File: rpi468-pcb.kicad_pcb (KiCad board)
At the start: 2 copper layers, 14 x 28.3 mm, 11 parts, among them J1 USB_A, J2 USB_C_Receptacle_USB2.0, J3 Conn_01x04_Female, U1 LM397

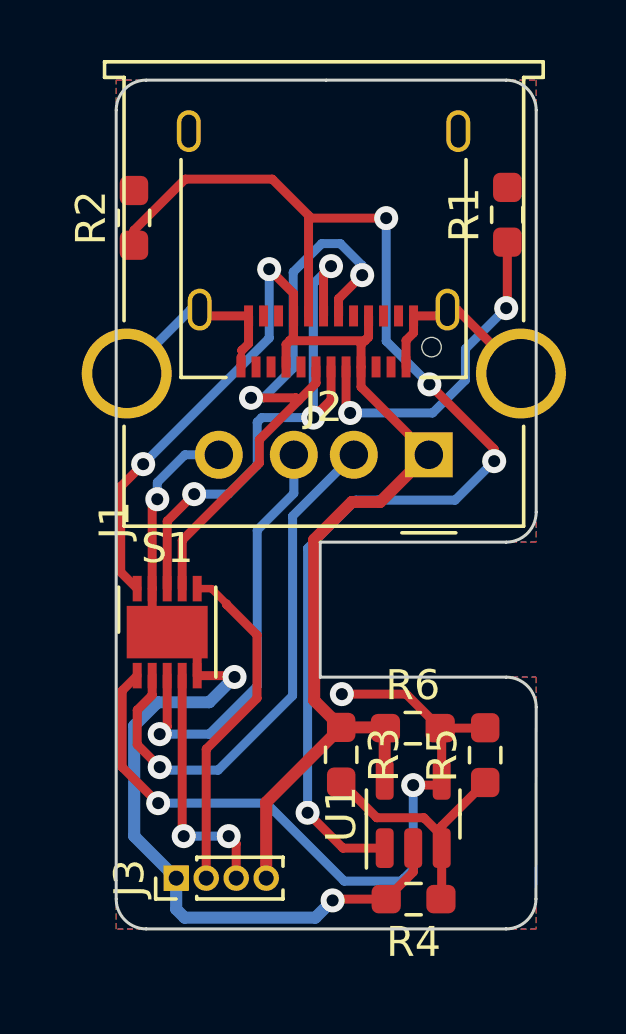
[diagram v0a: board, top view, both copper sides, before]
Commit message: some cleanup
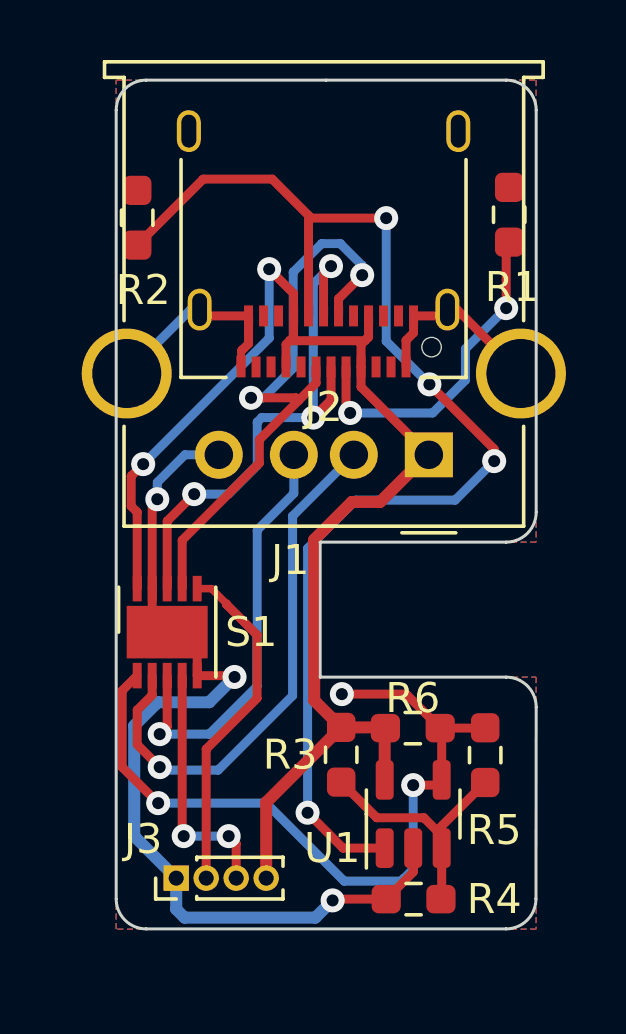
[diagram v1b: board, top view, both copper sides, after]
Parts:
- moved R2 0.11 mm to (164.7, 94.6)
- moved R1 0.06 mm to (177.1, 94.5)
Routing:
- net GND: track 44.5 -> 45.1 mm
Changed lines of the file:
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@@
     (property "Sheetname" "")
     (attr through_hole)
-    (fp_text reference "J3" (at 0 -1.56 90) (layer "F.SilkS")
+    (fp_text reference "J3" (at 1.3 -1.1 180) (layer "F.SilkS")
       (effects (font (size 1 1) (thickness 0.15)))
     )
@@
     (property "Sheetname" "")
     (attr smd)
-    (fp_text reference "R3" (at 0 -1.43 90) (layer "F.SilkS")
+    (fp_text reference "R3" (at 0 1.7 180) (layer "F.SilkS")
       (effects (font (size 1 1) (thickness 0.15)))
     )
@@
   )
   (footprint "Resistor_SMD:R_0603_1608Metric_Pad0.98x0.95mm_HandSolder" (layer "F.Cu")
-    (at 177.038 94.488 90)
+    (at 177.1 94.4875 90)
     (descr "Resistor SMD 0603 (1608 Metric), square (rectangular) end terminal, IPC_7351 nominal with elongated pad for handsoldering. (Body size source: IPC-SM-782 page 72, https://www.pcb-3d.com/wordpress/wp-content/uploads/ipc-sm-782a_amendment_1_and_2.pdf), generated with kicad-footprint-generator")
     (tags "resistor handsolder")
@@
     (property "Sheetname" "")
     (attr smd)
-    (fp_text reference "R1" (at 0 -1.43 90) (layer "F.SilkS")
+    (fp_text reference "R1" (at -2.4125 0.1 180) (layer "F.SilkS")
       (effects (font (size 1 1) (thickness 0.15)))
     )
@@
     (property "Sheetname" "")
     (attr smd)
-    (fp_text reference "R6" (at 0 -1.43) (layer "F.SilkS")
+    (fp_text reference "R6" (at 0 -1) (layer "F.SilkS")
       (effects (font (size 1 1) (thickness 0.15)))
     )
@@
     (property "Sheetname" "")
     (attr smd)
-    (fp_text reference "R5" (at 0 -1.43 90) (layer "F.SilkS")
+    (fp_text reference "R5" (at -2.5 0.3 180) (layer "F.SilkS")
       (effects (font (size 1 1) (thickness 0.15)))
     )
@@
     (property "Sheetname" "")
     (attr smd)
-    (fp_text reference "U1" (at 0 -2.4 90) (layer "F.SilkS")
+    (fp_text reference "U1" (at -1.1375 -2.7 180) (layer "F.SilkS")
       (effects (font (size 1 1) (thickness 0.15)))
     )
@@
     (property "Sheetname" "")
     (attr smd)
-    (fp_text reference "S1" (at 2.8 0 180) (layer "F.SilkS")
+    (fp_text reference "S1" (at 0 2.8 180) (layer "F.SilkS")
       (effects (font (size 1 1) (thickness 0.15)))
     )
@@
     (property "Sheetname" "")
     (attr smd)
-    (fp_text reference "R4" (at 0 -1.43) (layer "F.SilkS")
+    (fp_text reference "R4" (at -2.6875 0) (layer "F.SilkS")
       (effects (font (size 1 1) (thickness 0.15)))
     )
@@
     (property "Sheetname" "")
     (attr through_hole)
-    (fp_text reference "J1" (at 10.4733 -2.1792 90) (layer "F.SilkS")
+    (fp_text reference "J1" (at 4.6218 -3.511 180) (layer "F.SilkS")
       (effects (font (size 1 1) (thickness 0.15)))
     )
@@
       (effects (font (size 1 1) (thickness 0.15)))
     )
-    (fp_text user "${REFERENCE}" (at 3.5 3.7) (layer "F.Fab")
+    (fp_text user "${REFERENCE}" (at 4.6218 -3.511) (layer "F.Fab")
       (effects (font (size 1 1) (thickness 0.15)))
     )
@@
   )
   (footprint "Resistor_SMD:R_0603_1608Metric_Pad0.98x0.95mm_HandSolder" (layer "F.Cu")
-    (at 164.592 94.5915 90)
+    (at 164.7 94.5875 90)
     (descr "Resistor SMD 0603 (1608 Metric), square (rectangular) end terminal, IPC_7351 nominal with elongated pad for handsoldering. (Body size source: IPC-SM-782 page 72, https://www.pcb-3d.com/wordpress/wp-content/uploads/ipc-sm-782a_amendment_1_and_2.pdf), generated with kicad-footprint-generator")
     (tags "resistor handsolder")
@@
     (property "Sheetname" "")
     (attr smd)
-    (fp_text reference "R2" (at 0 -1.43 90) (layer "F.SilkS")
+    (fp_text reference "R2" (at -2.4125 0.2 180) (layer "F.SilkS")
       (effects (font (size 1 1) (thickness 0.15)))
     )
@@
   (gr_arc (start 178 104.4) (mid 177.707107 105.107107) (end 177 105.4) (layer "Edge.Cuts") (width 0.1))
   (gr_line (start 170.8 105.4) (end 170.8 109.9) (layer "Edge.Cuts") (width 0.1))
-  (gr_line (start 177 118.292893) (end 165 118.292893) (layer "Edge.Cuts") (width 0.1))
   (gr_line (start 170.8 109.9) (end 177 109.9) (layer "Edge.Cuts") (width 0.1))
   (gr_line (start 171 90) (end 165 90) (layer "Edge.Cuts") (width 0.1))
+  (gr_line (start 176.992893 118.292893) (end 165 118.292893) (layer "Edge.Cuts") (width 0.1))
   (gr_arc (start 177 109.9) (mid 177.707107 110.192893) (end 178 110.9) (layer "Edge.Cuts") (width 0.1))
   (gr_line (start 164 117.292893) (end 164 91) (layer "Edge.Cuts") (width 0.1))
@@
   (segment (start 169.785896 98.685896) (end 169.911792 98.56) (width 0.3) (layer "F.Cu") (net 1))
   (segment (start 169.785896 98.685896) (end 172.285896 98.685896) (width 0.3) (layer "F.Cu") (net 1))
+  (segment (start 164.5 103.2) (end 164.9 102.8) (width 0.3) (layer "F.Cu") (net 1))
   (segment (start 170.6 110.675) (end 171.5 111.575) (width 0.4) (layer "F.Cu") (net 1))
   (segment (start 169 116.6) (end 169 114.075) (width 0.4) (layer "F.Cu") (net 1))
@@
   (segment (start 172.95 111.625) (end 172.975 111.6) (width 0.4) (layer "F.Cu") (net 1))
   (segment (start 171.5 111.575) (end 172.95 111.575) (width 0.4) (layer "F.Cu") (net 1))
+  (segment (start 164.7 104.4) (end 164.5 104.2) (width 0.3) (layer "F.Cu") (net 1))
   (segment (start 169.661792 98.81) (end 169.785896 98.685896) (width 0.3) (layer "F.Cu") (net 1))
   (segment (start 169.1 96.3) (end 169.911792 97.111792) (width 0.3) (layer "F.Cu") (net 1))
-  (segment (start 164.15 103.55) (end 164.9 102.8) (width 0.3) (layer "F.Cu") (net 1))
+  (segment (start 164.5 104.2) (end 164.5 103.2) (width 0.3) (layer "F.Cu") (net 1))
   (segment (start 171.856357 104.0608) (end 170.6 105.317157) (width 0.4) (layer "F.Cu") (net 1))
-  (segment (start 164.7 106.95) (end 164.15 106.4) (width 0.3) (layer "F.Cu") (net 1))
   (segment (start 174.3718 102.489) (end 172.8 104.0608) (width 0.4) (layer "F.Cu") (net 1))
-  (segment (start 164.15 106.4) (end 164.15 103.55) (width 0.3) (layer "F.Cu") (net 1))
+  (segment (start 164.7 106.95) (end 164.7 104.4) (width 0.3) (layer "F.Cu") (net 1))
   (segment (start 169 114.075) (end 171.5 111.575) (width 0.4) (layer "F.Cu") (net 1))
   (segment (start 172.161792 99.56) (end 172.161792 98.81) (width 0.3) (layer "F.Cu") (net 1))
@@
   (segment (start 167.1 111.8) (end 165.4505 111.8) (width 0.3) (layer "B.Cu") (net 3))
   (segment (start 168.7 110.2) (end 167.1 111.8) (width 0.3) (layer "B.Cu") (net 3))
+  (segment (start 168.161792 99.56) (end 168.161792 99.025) (width 0.25) (layer "F.Cu") (net 4))
   (segment (start 173.661792 98.674999) (end 173.911792 98.424999) (width 0.3) (layer "F.Cu") (net 4))
   (segment (start 168.186792 99.013208) (end 168.186792 99) (width 0.3) (layer "F.Cu") (net 4))
@@
   (segment (start 174.831792 97.86) (end 175.041792 97.65) (width 0.3) (layer "F.Cu") (net 4))
   (segment (start 171.257076 117.3) (end 171.214385 117.342691) (width 0.3) (layer "F.Cu") (net 4))
+  (segment (start 168.161792 99.025) (end 168.186792 99) (width 0.25) (layer "F.Cu") (net 4))
   (segment (start 166.7 109.075) (end 166.7 109.85) (width 0.3) (layer "F.Cu") (net 4))
   (segment (start 168.411792 97.86) (end 168.411792 98.788208) (width 0.3) (layer "F.Cu") (net 4))
@@
   (segment (start 167.4218 102.489) (end 166.29043 102.489) (width 0.3) (layer "B.Cu") (net 4))
   (segment (start 166.781792 97.65) (end 166.4808 97.65) (width 0.3) (layer "B.Cu") (net 4))
-  (segment (start 177.038 95.4005) (end 177.038 97.562) (width 0.3) (layer "F.Cu") (net 5))
+  (segment (start 177 97.6) (end 177 95.5) (width 0.3) (layer "F.Cu") (net 5))
+  (segment (start 177 95.5) (end 177.1 95.4) (width 0.3) (layer "F.Cu") (net 5))
   (segment (start 171.661792 100.957092) (end 171.799548 101.094848) (width 0.3) (layer "F.Cu") (net 5))
   (segment (start 171.661792 99.56) (end 171.661792 100.957092) (width 0.3) (layer "F.Cu") (net 5))
@@
   (segment (start 173 94.6) (end 170.5 94.6) (width 0.3) (layer "F.Cu") (net 9))
   (segment (start 169.2 93.3) (end 170.411792 94.511792) (width 0.3) (layer "F.Cu") (net 9))
+  (segment (start 166.9 93.3) (end 169.2 93.3) (width 0.3) (layer "F.Cu") (net 9))
   (segment (start 176.6 102.7) (end 176.6 102.3) (width 0.3) (layer "F.Cu") (net 9))
-  (segment (start 166.3 93.3) (end 169.2 93.3) (width 0.3) (layer "F.Cu") (net 9))
   (segment (start 172.95 115.6) (end 171.559954 115.6) (width 0.3) (layer "F.Cu") (net 9))
-  (segment (start 164.592 95.008) (end 166.3 93.3) (width 0.3) (layer "F.Cu") (net 9))
+  (segment (start 164.7 95.5) (end 166.9 93.3) (width 0.3) (layer "F.Cu") (net 9))
   (segment (start 171.559954 115.6) (end 170.379977 114.420023) (width 0.3) (layer "F.Cu") (net 9))
-  (segment (start 164.592 95.504) (end 164.592 95.008) (width 0.3) (layer "F.Cu") (net 9))
   (segment (start 170.411792 94.511792) (end 170.411792 97.86) (width 0.3) (layer "F.Cu") (net 9))
   (via (at 174.440923 100.140923) (size 0.8) (drill 0.4) (layers "F.Cu" "B.Cu") (net 9))
